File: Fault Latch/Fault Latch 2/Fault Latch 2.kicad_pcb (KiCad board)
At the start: 2 copper layers, 89.6 x 111.1 mm, 107 parts, among them K101 Fujitsu_FTR-LYAA005x, K102 Fujitsu_FTR-LYAA005x, K103 Fujitsu_FTR-LYAA005x, Q101 Q_NPN_BEC, Q102 Q_NPN_BEC, Q103 Q_NPN_BEC, Q104 Q_NPN_BEC, Q105 Q_NMOS_GSD, Q106 Q_NMOS_GSD, Q107 Q_PMOS_GSD, Q108 Q_PMOS_GSD, Q109 Q_NMOS_GDS, Q110 Q_NPN_BEC, Q111 Q_NPN_BEC, Q112 Q_NMOS_GSD, Q113 Q_PMOS_GSD, SW101 SW_Omron_B3FS, SW102 SW_Omron_B3FS, SW103 SW_Omron_B3FS, U101 SFH617A-1, U102 SFH617A-1, U103 SFH617A-1, U104 74AHC1G00, U105 74AHC1G00, U106 74AHC1G00, U107 74LS279, U108 641964-1, U109 SFH617A-1, U110 SFH617A-1, U111 641964-1, U112 641964-1, U113 641964-1, U114 641964-1, U115 641964-1, U116 641964-1, U117 74AHC1G00, U118 LM555xM, U119 74AHC1G00, U120 641964-1, U121 SFH617A-1, U122 641964-1

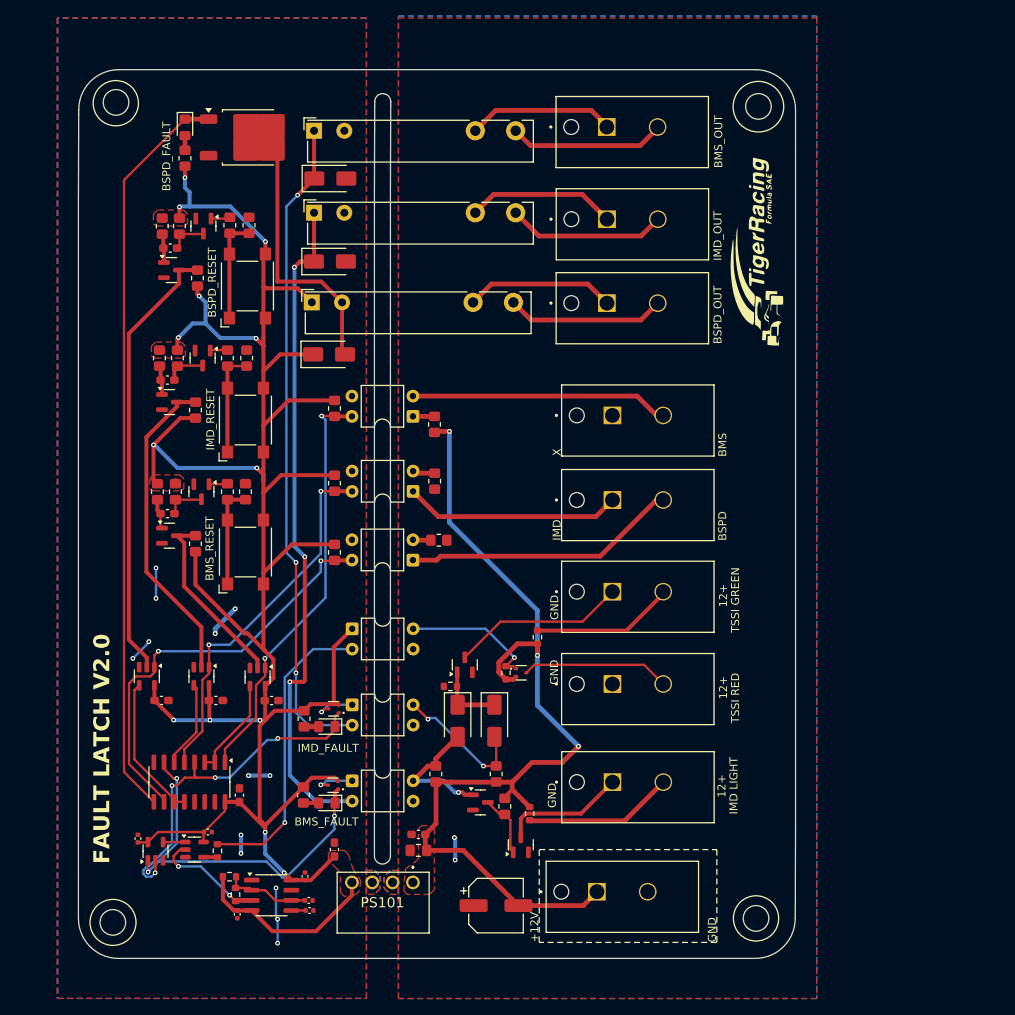
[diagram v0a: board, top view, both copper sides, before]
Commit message: FL READY
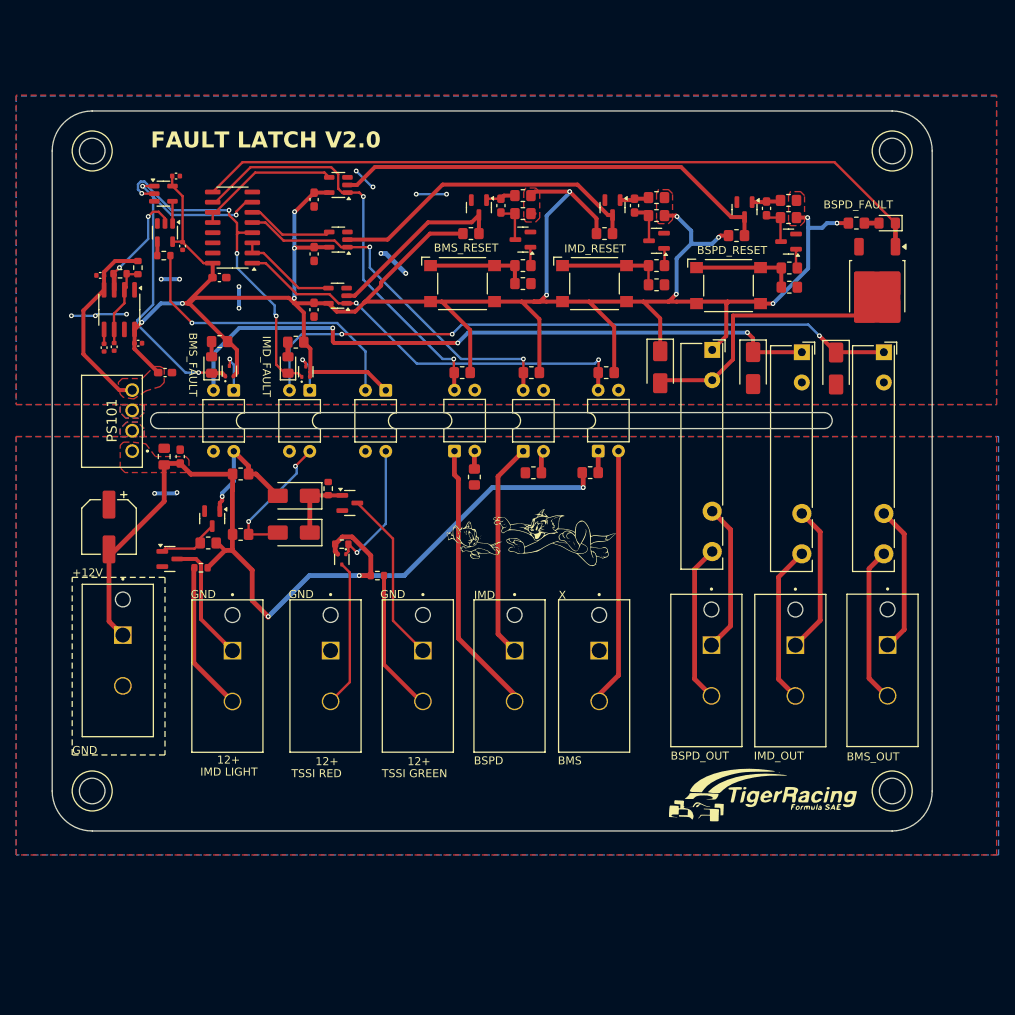
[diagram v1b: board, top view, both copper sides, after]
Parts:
- added G***: LOGO, LOGO, F.Cu at (128.3, 97.3)
- moved H104 97.2 mm to (174.2, 49.1), turned to -90 degrees
- moved H101 96.5 mm to (74.2, 49.1), turned to -90 degrees
- moved D103 88.6 mm to (173.6, 58.1), turned to 180 degrees
- moved H103 87.2 mm to (174.2, 129.1), turned to -90 degrees
- moved H102 84.5 mm to (74.2, 129.1), turned to -90 degrees
- moved R118 84.3 mm to (169.7, 58.1), turned to 180 degrees
- moved C110 82.9 mm to (84.7, 52.2), turned to 180 degrees
- moved U117 82.2 mm to (83.1, 54.4), turned to 0 degrees
- moved C108 81.7 mm to (75.2, 64.6), turned to 180 degrees
- moved Q109 80.7 mm to (172.3, 66.1), turned to -90 degrees
- moved R131 78.9 mm to (77.7, 64.4), turned to 0 degrees
- moved R127 78.4 mm to (161.3, 55.2), turned to 180 degrees
- moved U119 77.2 mm to (83.3, 59.3), turned to -90 degrees
- moved R132 77.0 mm to (79.9, 63.7), turned to 90 degrees
- moved K101 76.4 mm to (173.2, 74.2), turned to -90 degrees
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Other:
- board size 89.6 x 111.1 mm -> 110 x 90 mm
